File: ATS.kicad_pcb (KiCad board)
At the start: 2 copper layers, 72.3 x 37.7 mm, 15 parts

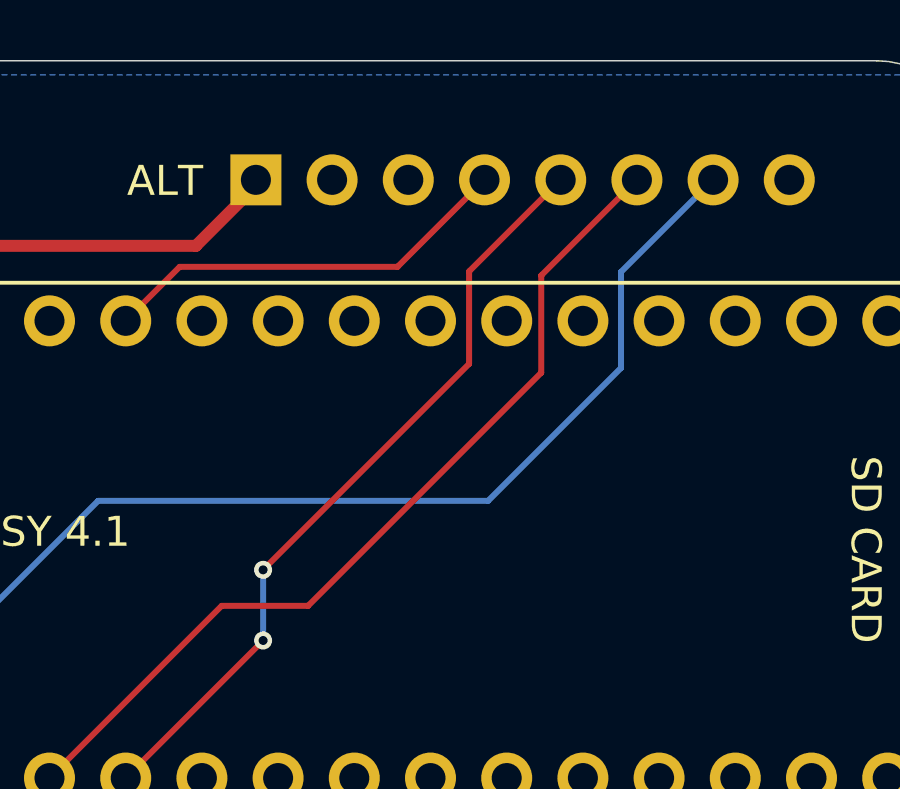
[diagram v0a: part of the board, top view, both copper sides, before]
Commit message: incorporated libraries
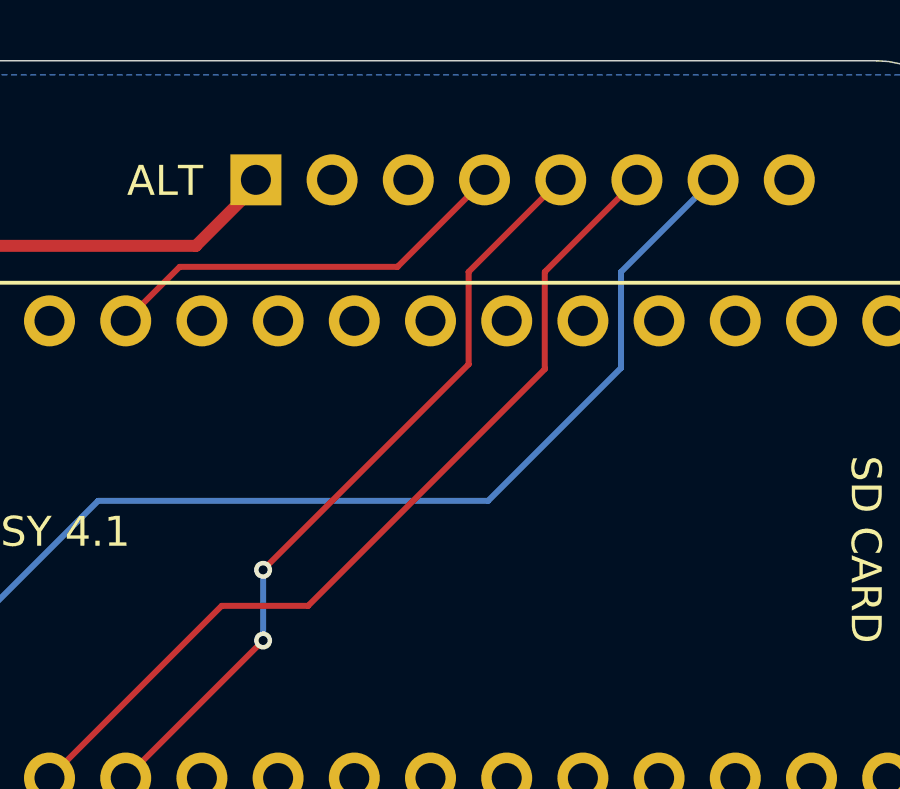
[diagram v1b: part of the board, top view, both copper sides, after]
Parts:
- ADAFRUITBUZZER_1: footprint CPT-2212-3TH:adafruit -> AdafruitBuzzer:AdafruitBuzzer
- TEENSY4.1_1: footprint DEV-16771:MODULE_DEV-16771 -> Teensy4.1:Teensy4.1
